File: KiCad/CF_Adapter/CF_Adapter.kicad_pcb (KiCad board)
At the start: 2 copper layers, 27 x 53.3 mm, 3 parts, among them J1 Z-Fighter IDE Connector, J2 Conn_02x25_Top_Bottom

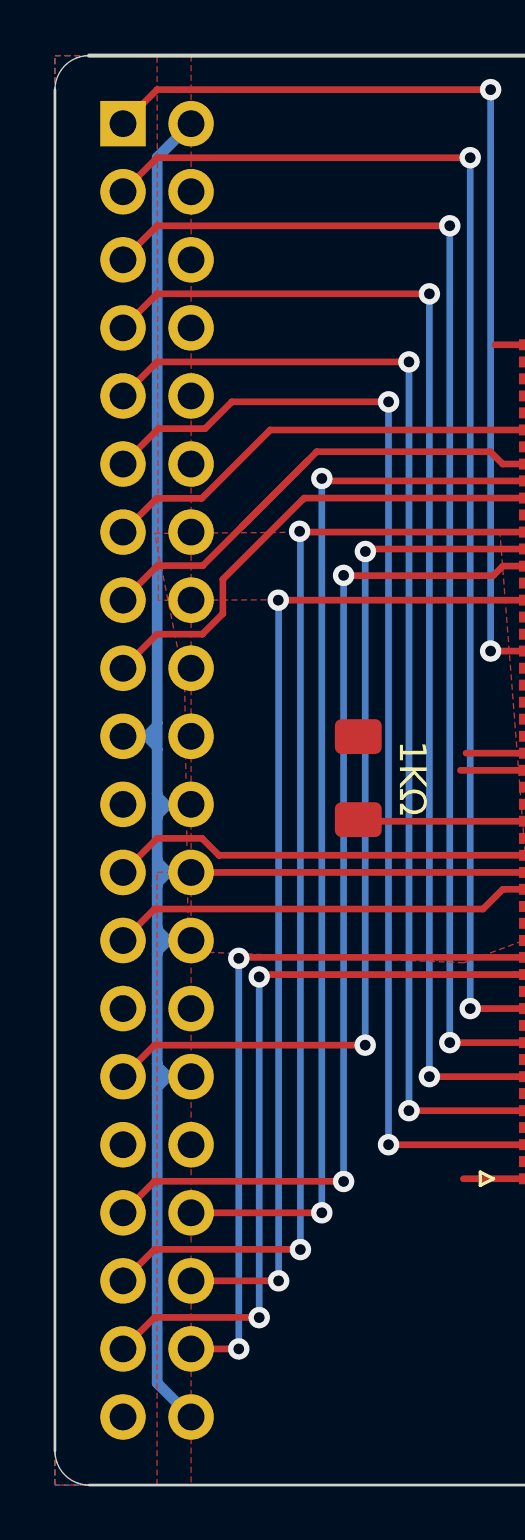
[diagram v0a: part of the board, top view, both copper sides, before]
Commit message: Routing
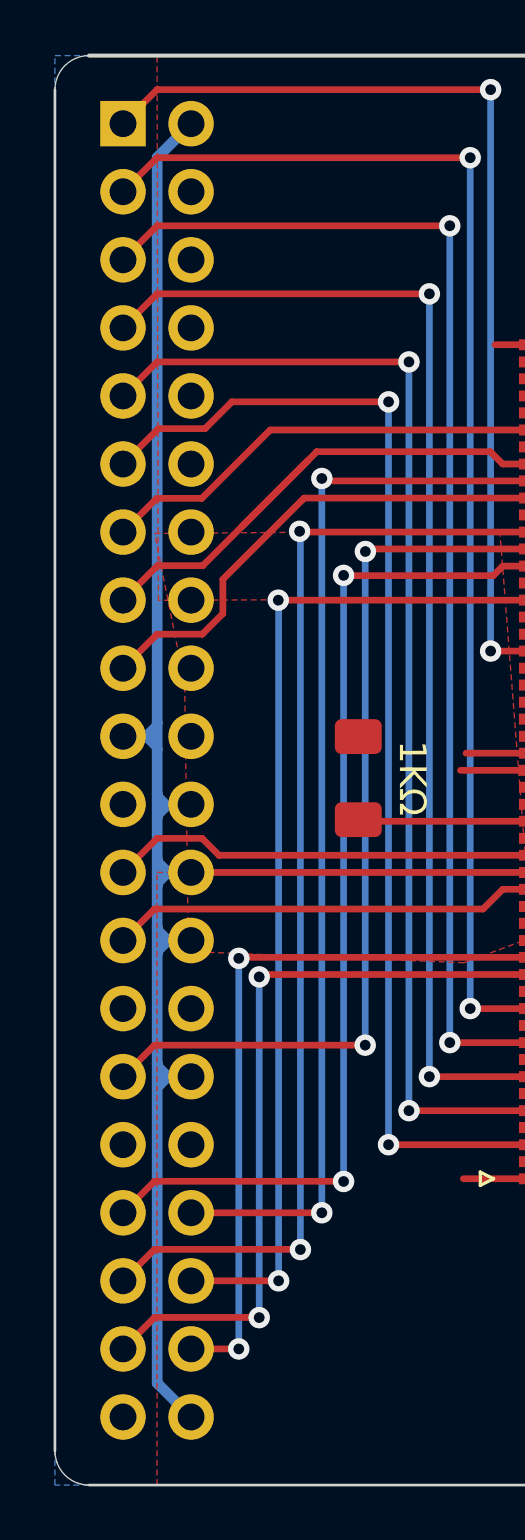
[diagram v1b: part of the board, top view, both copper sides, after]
